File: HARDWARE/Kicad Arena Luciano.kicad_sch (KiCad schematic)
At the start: 46 parts, among them IC1 MC7805CD2TG, J1 BORNERA, J2 BORNERA, J4 BORNERA, J5 BORNERA, K3 SANYOU_SRD_Form_C, K6 SANYOU_SRD_Form_C, K7 SANYOU_SRD_Form_C, K8 SANYOU_SRD_Form_C, Q1 BC547, Q2 BC547, Q4 BC547, Q5 BC547, SW1 SWITCH, U1 PC81713NIP0X, U2 PC81713NIP0X, U4 PC81713NIP0X, U5 PC81713NIP0X, U7 ESP32-DEVKITC

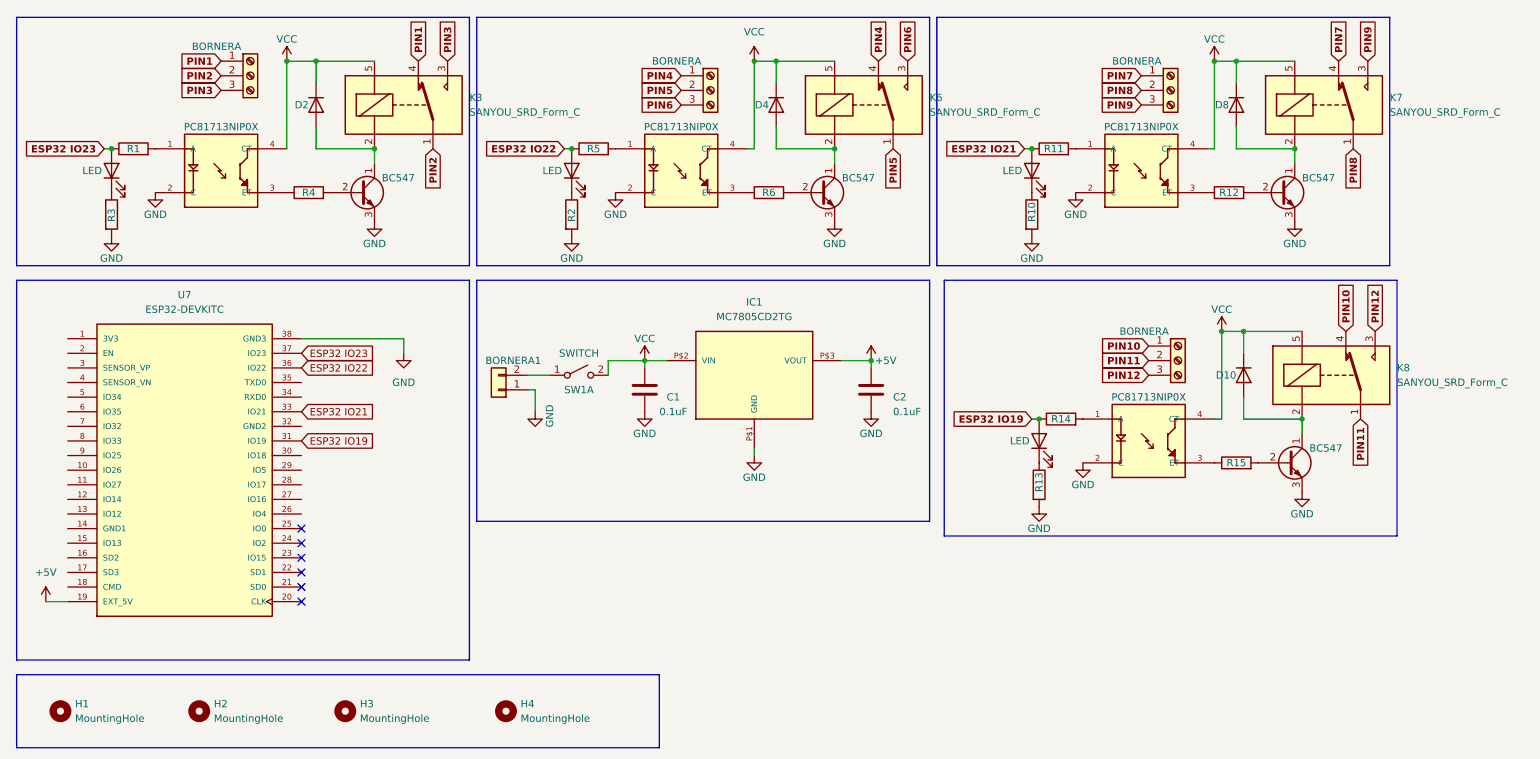
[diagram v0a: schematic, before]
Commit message: comi2
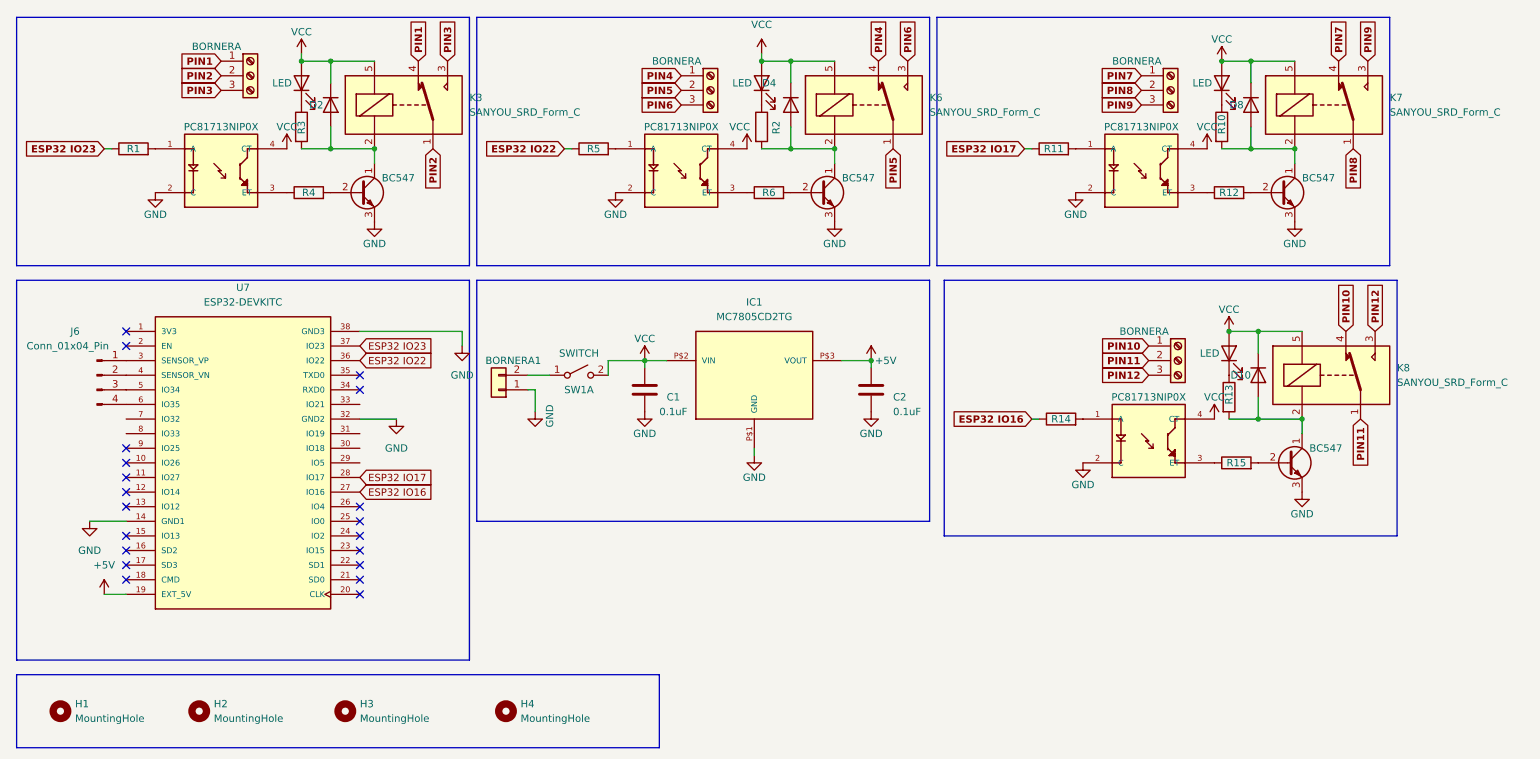
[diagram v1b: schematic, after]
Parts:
- added J6: Conn_01x04_Pin, Connector_PinHeader_2.54mm:PinHeader_1x04_P2.54mm_Vertical, symbol Connector:Conn_01x04_Pin
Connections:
- net ESP32 IO22: no longer D1.2 (A)
- net ESP32 IO23: no longer D3.2 (A)
- net GND: now also U7.14 (GND1), U7.32 (GND2); no longer R10.2, R13.2, R2.2, R3.2
- net VCC: now also D1.2 (A), D3.2 (A), D7.2 (A), D9.2 (A)
- net at D10.2 (A), K8.2, Q5.1 (C): now also R13.2
- net at D8.2 (A), K7.2, Q4.1 (C): now also R10.2
- net at D2.2 (A), K3.2, Q2.1 (C): now also R3.2
- net at D4.2 (A), K6.2, Q1.1 (C): now also R2.2
- net ESP32 IO16: now reaches U7.27 (IO16)
- net ESP32 IO16: now also R14.1
- net ESP32 IO17: now reaches U7.28 (IO17)
- net at U7.3 (SENSOR_VP): now also J6.1 (Pin_1)
- net at U7.4 (SENSOR_VN): now also J6.2 (Pin_2)
- net at U7.5 (IO34): now also J6.3 (Pin_3)
- net at U7.6 (IO35): now also J6.4 (Pin_4)
- net  ESP32 IO21 renamed  ESP32 IO17
- net  ESP32 IO17: no longer D7.2 (A)
- removed net ESP32 IO19: D9.2 (A), R14.1, U7.31 (IO19)
- net ESP32 IO21: no longer names the net of U7.33 (IO21)
- no-connect marks 6 -> 20
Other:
- moved on the sheet: D10, D2, D4, D8, R10, R13, R2, R3, U7
